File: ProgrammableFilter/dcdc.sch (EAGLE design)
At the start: 17 parts, among them IC1 MC34063AP, X1 22-23-2021, X2 22-23-2021

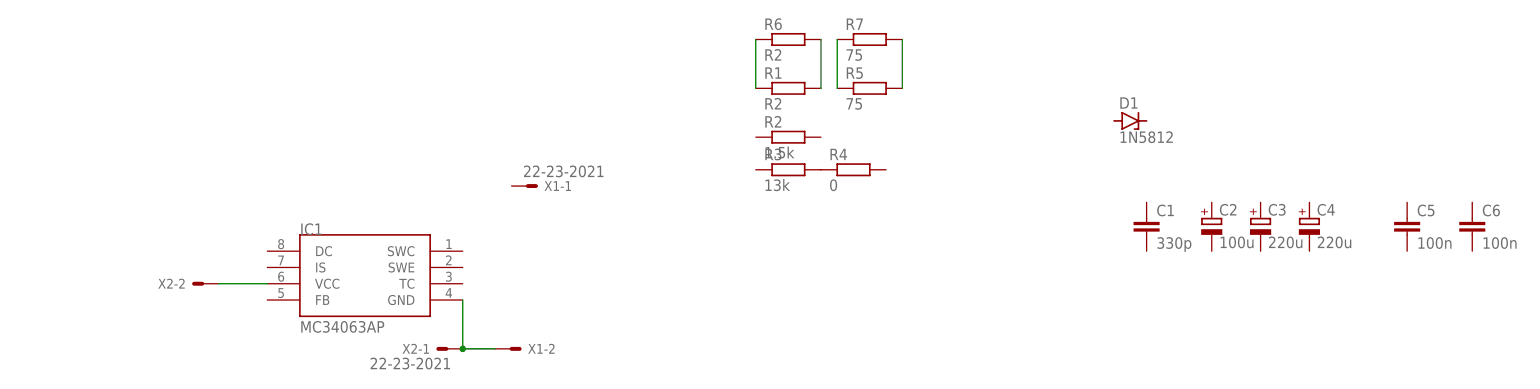
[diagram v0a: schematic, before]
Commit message: a
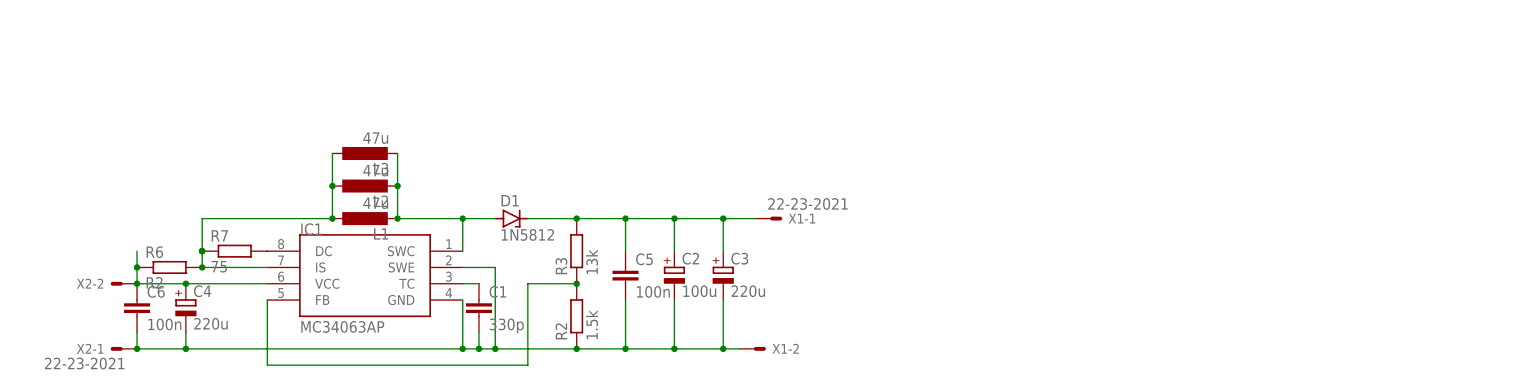
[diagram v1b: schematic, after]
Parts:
- removed R1: R2, rcl:R-EU_0207/10
- removed R4: 0, rcl:R-EU_R0805
- removed R5: 75, rcl:R-EU_0207/10
- added L1: 47u, rcl:L-EUTJ3-U2
- added L2: 47u, rcl:L-EUTJ4-U2
- added L3: 47u, rcl:L-EU6000-XXX-RC
- C2, C3, C4: device rcl:CPOL-EUE5-10.5 -> rcl:CPOL-EUE5-8.5
- R3: device rcl:R-EU_R0805 -> rcl:R-EU_0204/7
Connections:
- removed net N$1: R3.2, R4.1
- removed net N$2: R1.1, R6.1
- removed net N$4: R5.1, R7.1
- removed net N$6: IC1.GND, X1-2.S, X2-1.S
- removed net N$7: IC1.VCC, X2-2.S
- new net FB: IC1.FB, R2.2, R3.1
- new net GND: C1.2, C2.-, C3.-, C4.-, C5.2, C6.2, IC1.GND, IC1.SWE, R2.1, X1-2.S, X2-1.S
- new net N$9: C1.1, IC1.TC
- new net SW: D1.A, IC1.SWC, L1.2, L2.2, L3.2
- new net VIN: C4.+, C6.1, IC1.VCC, R6.1, X2-2.S
- new net VOUT: C2.+, C3.+, C5.1, D1.C, R3.2, X1-1.S
- net N$3: now also IC1.DC, R7.2; no longer R1.2, R6.2
- net N$5: now also IC1.IS, L1.1, L2.1, L3.1, R6.2, R7.1; no longer R5.2, R7.2
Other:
- moved on the sheet: C1, C2, C3, C4, C5, C6, D1, R2, R3, R6, R7, X1-1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
